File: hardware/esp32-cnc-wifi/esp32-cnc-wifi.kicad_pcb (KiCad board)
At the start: 2 copper layers, 52.1 x 52.1 mm, 12 parts, among them J1 HSPI, J2 Prog, U1 ESP-32S, U2 TXS0102-DIL, U3 AP1117-15

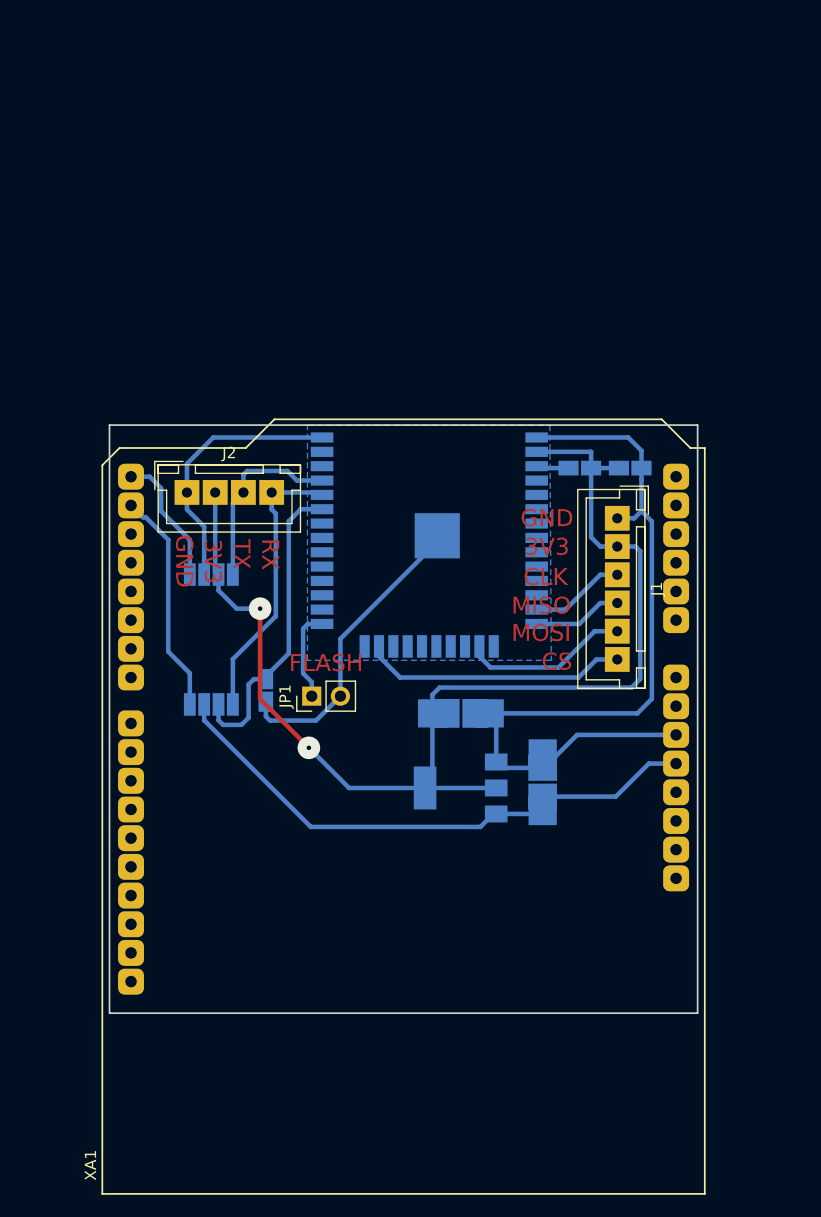
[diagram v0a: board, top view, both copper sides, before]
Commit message: Rotating board by 90-degrees.
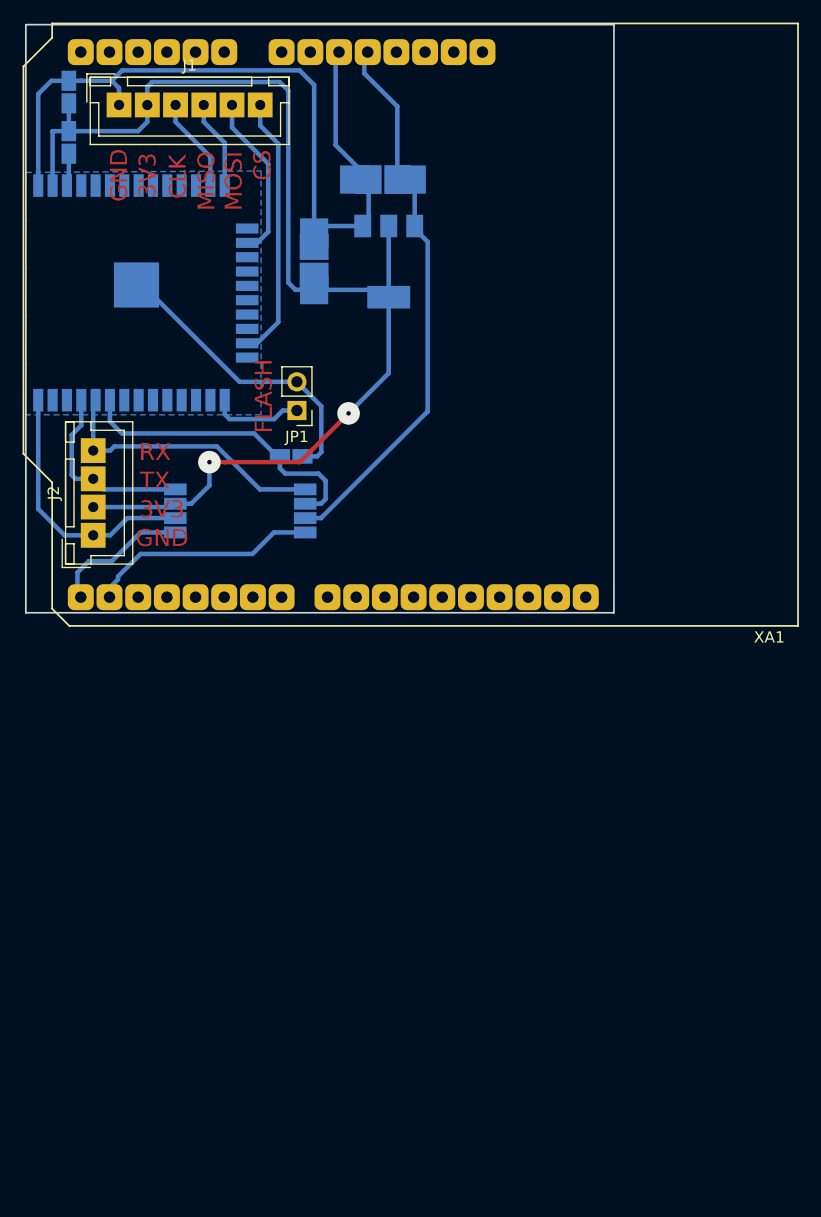
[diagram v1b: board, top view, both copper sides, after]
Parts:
- moved XA1 104.0 mm to (177.8, 38.1), turned to 180 degrees
- moved C1 59.8 mm to (113.2, 44.2), turned to 270 degrees
- moved J1 57.3 mm to (117.7, 45.3), turned to 0 degrees
- moved C2 55.2 mm to (141.1, 51.9), turned to 180 degrees
- moved R1 53.6 mm to (113.2, 48.6), turned to 90 degrees
- moved U3 47.0 mm to (141.6, 59.2), turned to 270 degrees
- moved C3 42.1 mm to (135.0, 59.2), turned to 90 degrees
- moved U1 34.5 mm to (115.8, 62.0), turned to 0 degrees
- moved JP1 25.3 mm to (133.4, 72.4), turned to 180 degrees
- moved R2 20.8 mm to (132.9, 76.4), turned to 180 degrees
- moved U2 10.8 mm to (128.1, 81.9), turned to 0 degrees
- moved J2 9.12 mm to (115.4, 83.4), turned to 90 degrees
